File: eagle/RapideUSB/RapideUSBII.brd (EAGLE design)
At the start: 50 x 24.6 mm, 40 parts, among them Q1 12MHz

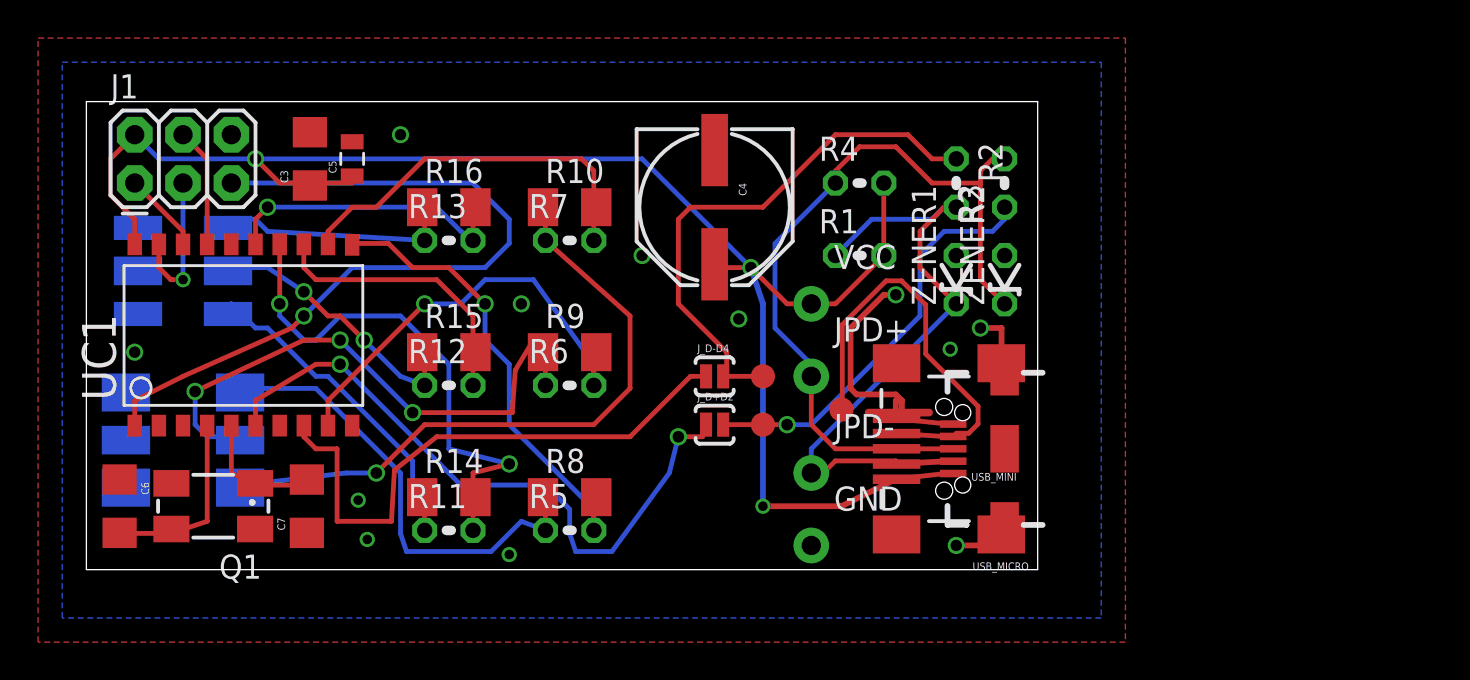
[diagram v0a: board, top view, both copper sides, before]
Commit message: Before routing
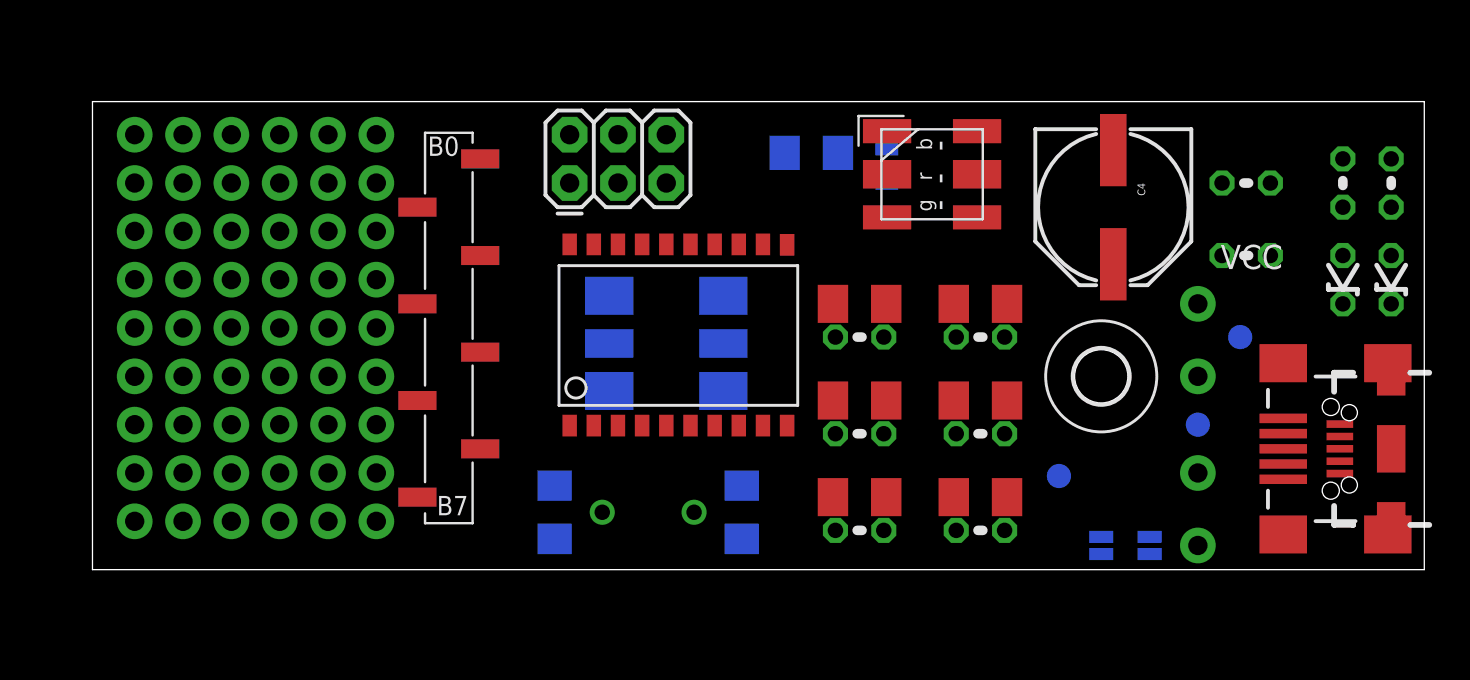
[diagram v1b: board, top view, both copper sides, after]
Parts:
- added H1: MOUNT-HOLE2.8, holes:2,8
- added J10: (no value), SparkFun-Connectors:1X08_SMD
- added J2, J4, J5, J6, J7, J8: (no value), SparkFun-Connectors:1X08_NO_SILK
- added J3: (no value), SparkFun-Connectors:1X08_SMD_ALT
- added J9: (no value), SparkFun-Connectors:1X06_NO_SILK
- Q1: device crystal:CTS406 -> SparkFun-Clocks:HC49U
- moved LED2 44.7 mm to (47.0, 18.4), flipped to the top
- moved C5 28.1 mm to (42.1, 21.3), flipped to the bottom
- moved C3 26.4 mm to (38.1, 21.9), flipped to the bottom, turned to 180 degrees
- moved LED1 25.9 mm to (30.5, 8.89)
- moved J_D-D4 24.5 mm to (55.9, 1.27), flipped to the bottom, turned to 90 degrees
- moved JP_D- 23.0 mm to (58.4, 7.62), flipped to the bottom
- moved C6 22.9 mm to (24.6, 3.02), flipped to the bottom, turned to 90 degrees
- moved C7 22.9 mm to (34.4, 3.02), flipped to the bottom, turned to 270 degrees
- moved Q1 22.9 mm to (29.5, 3.02), flipped to the bottom, turned to 0 degrees
- moved J1 22.9 mm to (25.4, 20.3)
- moved U$1 22.9 mm to (51.1, 1.27)
- moved UC1 22.9 mm to (30.5, 12.7)
- moved R10 22.2 mm to (47.0, 14.0)
- moved R7 22.2 mm to (47.0, 12.2)
- moved R13 22.2 mm to (40.6, 12.2)
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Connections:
- net D0: now also J10.8
- net D1: now also J10.7
- net D2: now also J10.6
- net D3: now also J10.5
- net D4: now also J10.4
- net GND: now also J9.1, J9.2, J9.3
- net LED1B: now also J3.8
- net LED1G: now also J10.2
- net LED1R: now also J10.3
- net LED2B: now also J3.5
- net LED2G: now also J3.6
- net LED2R: now also J3.7
- net MISO: now also J3.2
- net MOSI: now also J3.3
- net N$1: now also J3.4
- net N$23: now also Q1.2; no longer Q1.3
- net SCK: now also J3.1
- net VCC: now also J9.4, J9.5, J9.6
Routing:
- net VCC: track 85.7 -> 0.00 mm, vias 3 -> 0
- net USBD+: track 41.4 -> 0.00 mm
- net RESET: track 40.3 -> 0.00 mm, vias 1 -> 0
- net D2: track 34.9 -> 0.00 mm, vias 2 -> 0
- net N$18: track 34.1 -> 0.00 mm, vias 1 -> 0
- net USBD-: track 31.4 -> 0.00 mm
- net D4: track 30.3 -> 0.00 mm
- net N$17: track 30.1 -> 0.00 mm, vias 3 -> 0
- net D-: track 28.4 -> 0.00 mm
- net LED2G: track 27.6 -> 0.00 mm, vias 2 -> 0
- net LED1G: track 24.5 -> 0.00 mm, vias 1 -> 0
- net N$15: track 24.5 -> 0.00 mm
- net LED1R: track 23.2 -> 0.00 mm, vias 1 -> 0
- net D+: track 21.8 -> 0.00 mm, vias 1 -> 0
- net GND: track 21.3 -> 0.00 mm, vias 12 -> 0
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- removed copper zone on layer 1, net GND
- removed copper zone on layer 16, net GND
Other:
- board size 50 x 24.6 mm -> 70 x 24.6 mm
- board text added: "B0"
- board text added: "B7"
- board text added: "D0"
- board text added: "D6"
- board text added: "NC"
